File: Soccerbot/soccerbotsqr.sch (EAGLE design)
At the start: 37 parts, among them X1 NXT-SOCKET, X2 NXT-SOCKET, X3 NXT-SOCKET, X4 NXT-SOCKET, X5 NXT-SOCKET, X6 NXT-SOCKET, X7 NXT-SOCKET, X8 NXT-SOCKET

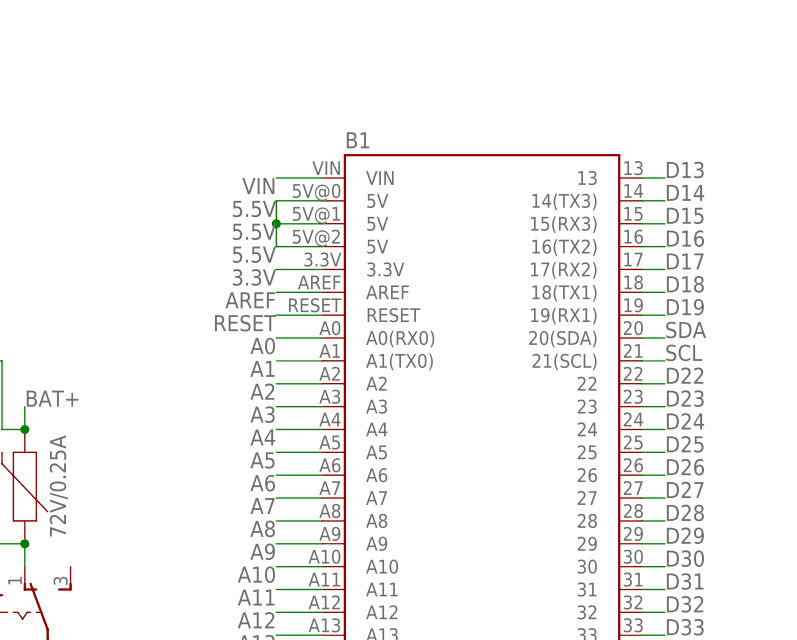
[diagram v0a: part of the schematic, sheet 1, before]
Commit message: dfg
dfg
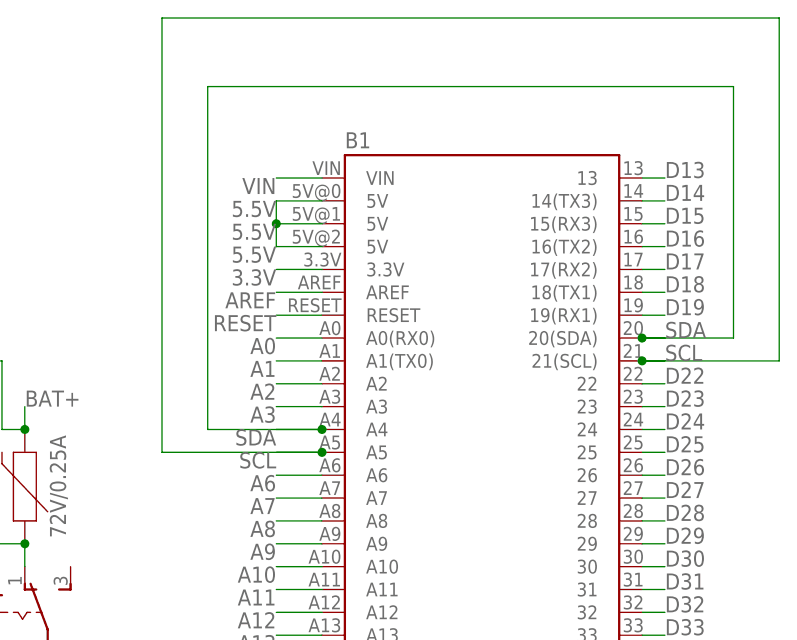
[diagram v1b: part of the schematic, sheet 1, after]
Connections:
- removed net A4: B1.A4
- removed net A5: B1.A5
- net SCL: now also B1.A5
- net SDA: now also B1.A4
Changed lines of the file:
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@@
 <?xml version="1.0" encoding="utf-8"?>
 <!DOCTYPE eagle SYSTEM "eagle.dtd">
-<eagle version="8.0.0">
+<eagle version="8.3.0">
 <drawing>
 <settings>
 <setting alwaysvectorfont="no"/>
+<setting keepoldvectorfont="yes"/>
 <setting verticaltext="up"/>
 </settings>
@@
 </segment>
 </net>
-<net name="A4" class="0">
-<segment>
-<pinref part="B1" gate="G$1" pin="A4"/>
-<wire x1="-154.94" y1="96.52" x2="-160.02" y2="96.52" width="0.1524" layer="91"/>
-<label x="-160.02" y="96.52" size="1.778" layer="95" rot="R180"/>
-</segment>
-</net>
 <net name="D1" class="0">
 <segment>
@@
 </segment>
 </net>
-<net name="SDA" class="0">
-<segment>
-<pinref part="B1" gate="G$1" pin="20(SDA)"/>
-<wire x1="-119.38" y1="106.68" x2="-116.84" y2="106.68" width="0.1524" layer="91"/>
-<label x="-116.84" y="106.68" size="1.778" layer="95"/>
-</segment>
-</net>
 <net name="SCL" class="0">
 <segment>
@@
 <wire x1="-119.38" y1="104.14" x2="-116.84" y2="104.14" width="0.1524" layer="91"/>
 <label x="-116.84" y="104.14" size="1.778" layer="95"/>
+<wire x1="-119.38" y1="104.14" x2="-104.14" y2="104.14" width="0.1524" layer="91"/>
+<wire x1="-104.14" y1="104.14" x2="-104.14" y2="142.24" width="0.1524" layer="91"/>
+<junction x="-119.38" y="104.14"/>
+<wire x1="-104.14" y1="142.24" x2="-172.72" y2="142.24" width="0.1524" layer="91"/>
+<wire x1="-172.72" y1="142.24" x2="-172.72" y2="93.98" width="0.1524" layer="91"/>
+<pinref part="B1" gate="G$1" pin="A5"/>
+<wire x1="-154.94" y1="93.98" x2="-160.02" y2="93.98" width="0.1524" layer="91"/>
+<label x="-160.02" y="93.98" size="1.778" layer="95" rot="R180"/>
+<wire x1="-172.72" y1="93.98" x2="-154.94" y2="93.98" width="0.1524" layer="91"/>
+<junction x="-154.94" y="93.98"/>
 </segment>
 </net>
@@
 </segment>
 </net>
-<net name="A5" class="0">
-<segment>
-<pinref part="B1" gate="G$1" pin="A5"/>
-<wire x1="-154.94" y1="93.98" x2="-160.02" y2="93.98" width="0.1524" layer="91"/>
-<label x="-160.02" y="93.98" size="1.778" layer="95" rot="R180"/>
-</segment>
-</net>
 <net name="D44" class="0">
 <segment>
@@
 </segment>
 </net>
+<net name="SDA" class="0">
+<segment>
+<pinref part="B1" gate="G$1" pin="A4"/>
+<wire x1="-154.94" y1="96.52" x2="-160.02" y2="96.52" width="0.1524" layer="91"/>
+<label x="-160.02" y="96.52" size="1.778" layer="95" rot="R180"/>
+<wire x1="-154.94" y1="96.52" x2="-167.64" y2="96.52" width="0.1524" layer="91"/>
+<wire x1="-167.64" y1="96.52" x2="-167.64" y2="134.62" width="0.1524" layer="91"/>
+<junction x="-154.94" y="96.52"/>
+<wire x1="-167.64" y1="134.62" x2="-109.22" y2="134.62" width="0.1524" layer="91"/>
+<wire x1="-109.22" y1="134.62" x2="-109.22" y2="106.68" width="0.1524" layer="91"/>
+<pinref part="B1" gate="G$1" pin="20(SDA)"/>
+<wire x1="-119.38" y1="106.68" x2="-116.84" y2="106.68" width="0.1524" layer="91"/>
+<label x="-116.84" y="106.68" size="1.778" layer="95"/>
+<wire x1="-109.22" y1="106.68" x2="-119.38" y2="106.68" width="0.1524" layer="91"/>
+<junction x="-119.38" y="106.68"/>
+</segment>
+</net>
